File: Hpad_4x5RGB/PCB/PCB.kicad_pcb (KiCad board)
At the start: 2 copper layers, 113.2 x 73.7 mm, 128 parts, among them J1 AVR-ISP-6, J10 Conn_4P_FM, J2 1x1_fm, J3 1x1_fm, J4 Conn_4P_FM, J5 Conn_4P_FM, J6 1x1_fm, J7 1x1_fm, J8 Conn_4P_FM, J9 01x05_fm, Q1 PZT2222A, SW1 Bootloader, SW10 SW_Push, SW11 SW_Push, SW12 SW_Push, SW13 SW_Push, SW14 SW_Push, SW15 SW_Push, SW16 SW_Push, SW17 SW_Push, SW18 SW_Push, SW19 SW_Push, SW2 SW_Push, SW20 SW_Push, SW21 SW_Push, SW22 SW_Push, SW23 SW_Push, SW24 SW_Push, SW25 SW_Push, SW26 SW_Push, SW27 SW_Push, SW28 SW_Push, SW3 SW_Push, SW4 SW_Push, SW5 SW_Push, SW6 SW_Push, SW7 SW_Push, SW8 SW_Push, SW9 SW_Push, U1 ATmega32U4-MU, U2 AP1117-50, U3 WS2811, Y1 16mhz

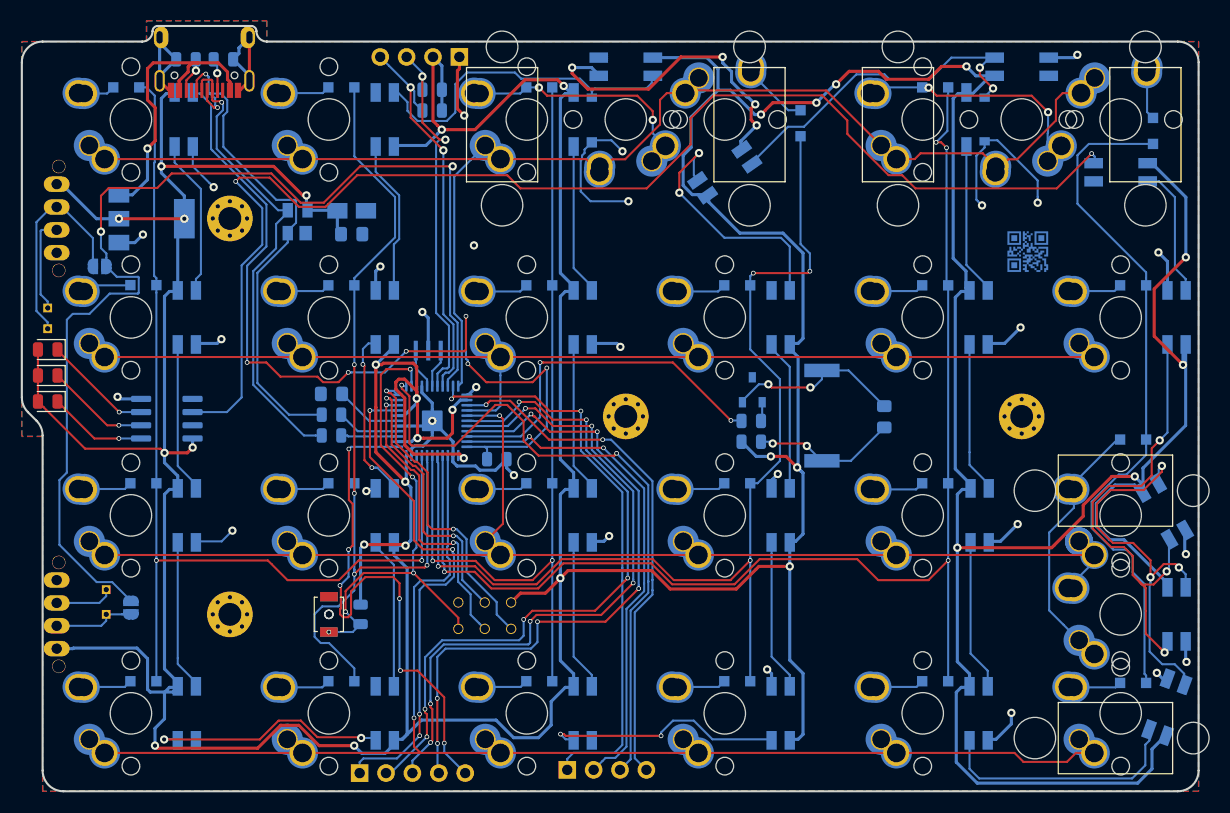
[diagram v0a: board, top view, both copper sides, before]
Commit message: missing wire fix
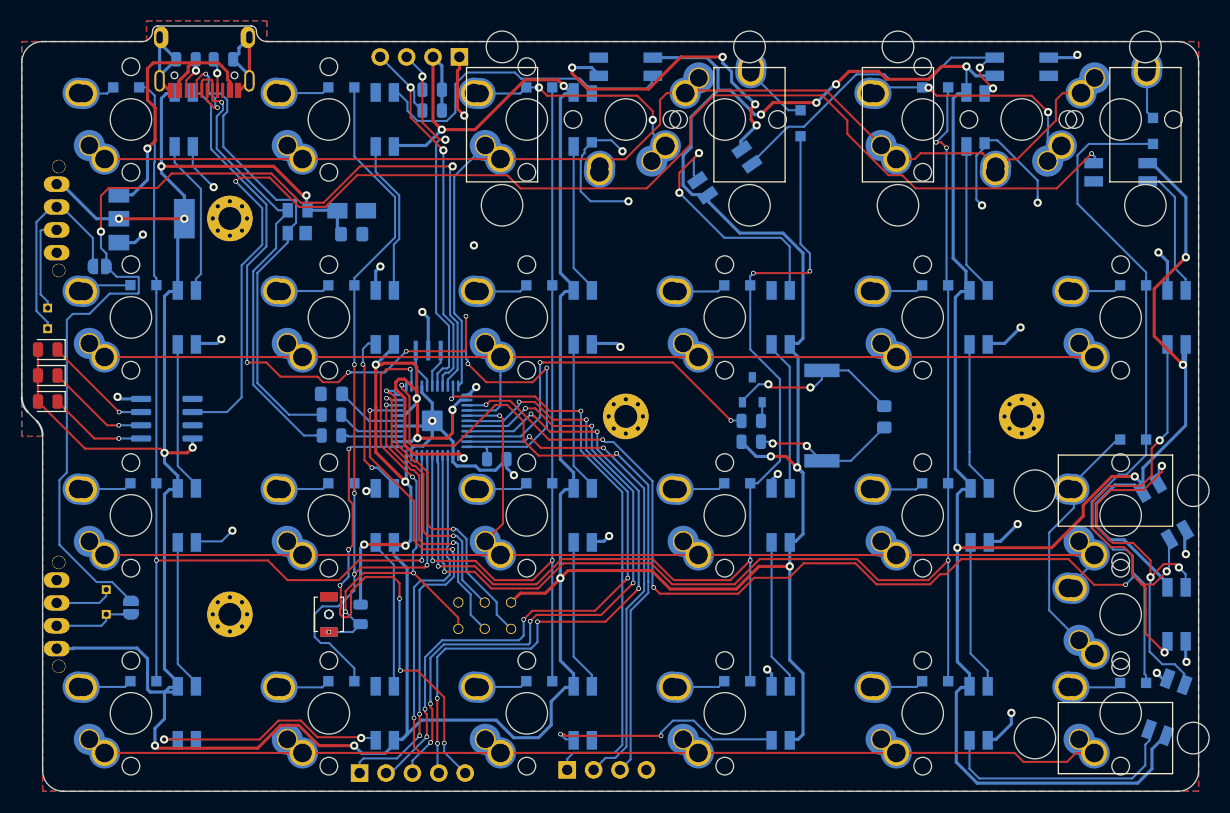
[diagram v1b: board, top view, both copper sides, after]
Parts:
- removed G***: LOGO, Footprint_hnah87:QR_code-m-me-HnahKB_solder_mask
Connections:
- J10 pad 4: D4 -> GND
- U1 pad 25: D4 -> Row6
- U1 pad 42: (no net) -> Net-(U1-Pad42)
- U3 pad 5: (no net) -> RGB_Data-OUT
- U3 pad 7: (no net) -> Net-(U3-Pad7)
- USB1 pad 3: (no net) -> Net-(USB1-Pad3)
- USB1 pad 9: (no net) -> Net-(USB1-Pad9)
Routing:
- net Row6: track 66.7 -> 149.5 mm, vias 0 -> 4
- net D4: track 50.2 -> 0.00 mm, vias 2 -> 0
- net VCC: track 716.3 -> 715.4 mm
